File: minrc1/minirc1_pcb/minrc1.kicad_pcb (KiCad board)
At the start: 2 copper layers, 39 x 49.5 mm, 18 parts, among them J3 Conn_01x04, J4 Conn_01x04, U1 DRV8837D, U2 DRV8837D, U3 DRV8837D, U4 DRV8837D, U5 ESP32S3

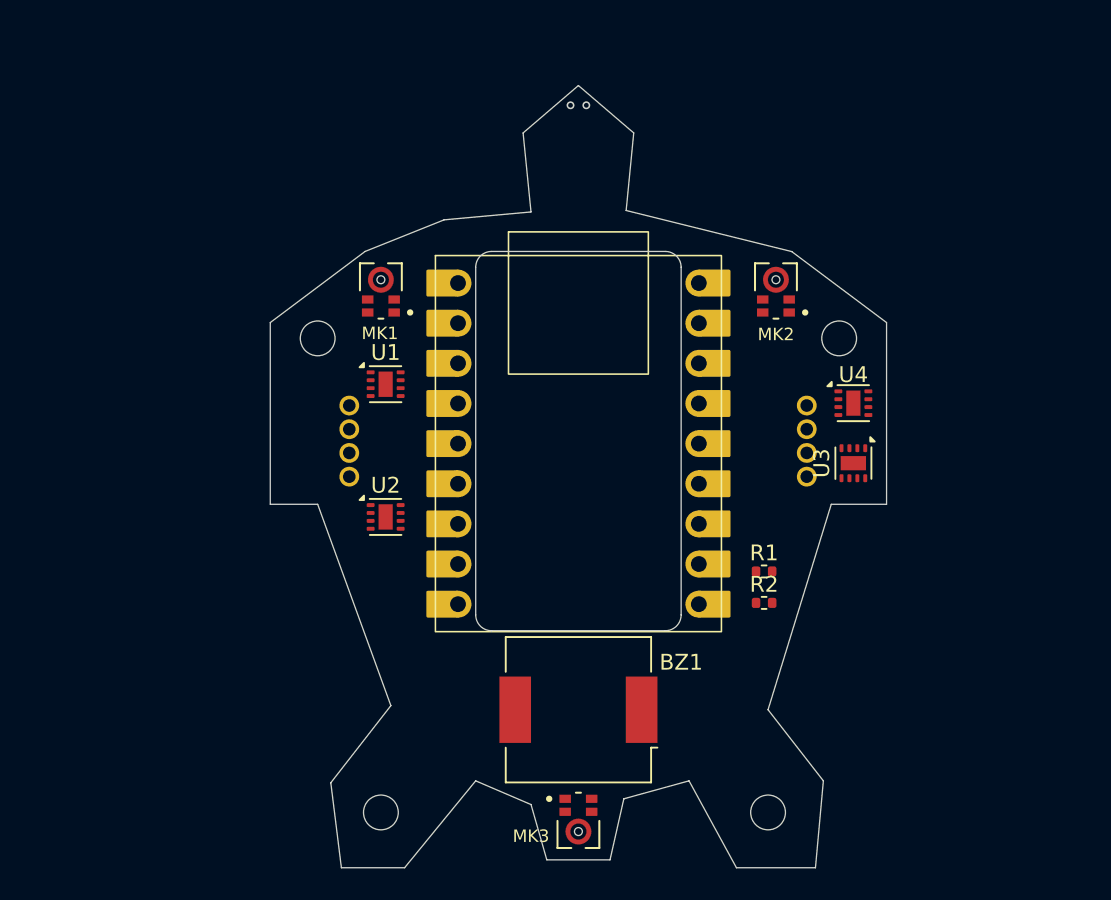
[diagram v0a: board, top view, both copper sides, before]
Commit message: finish turtlebot
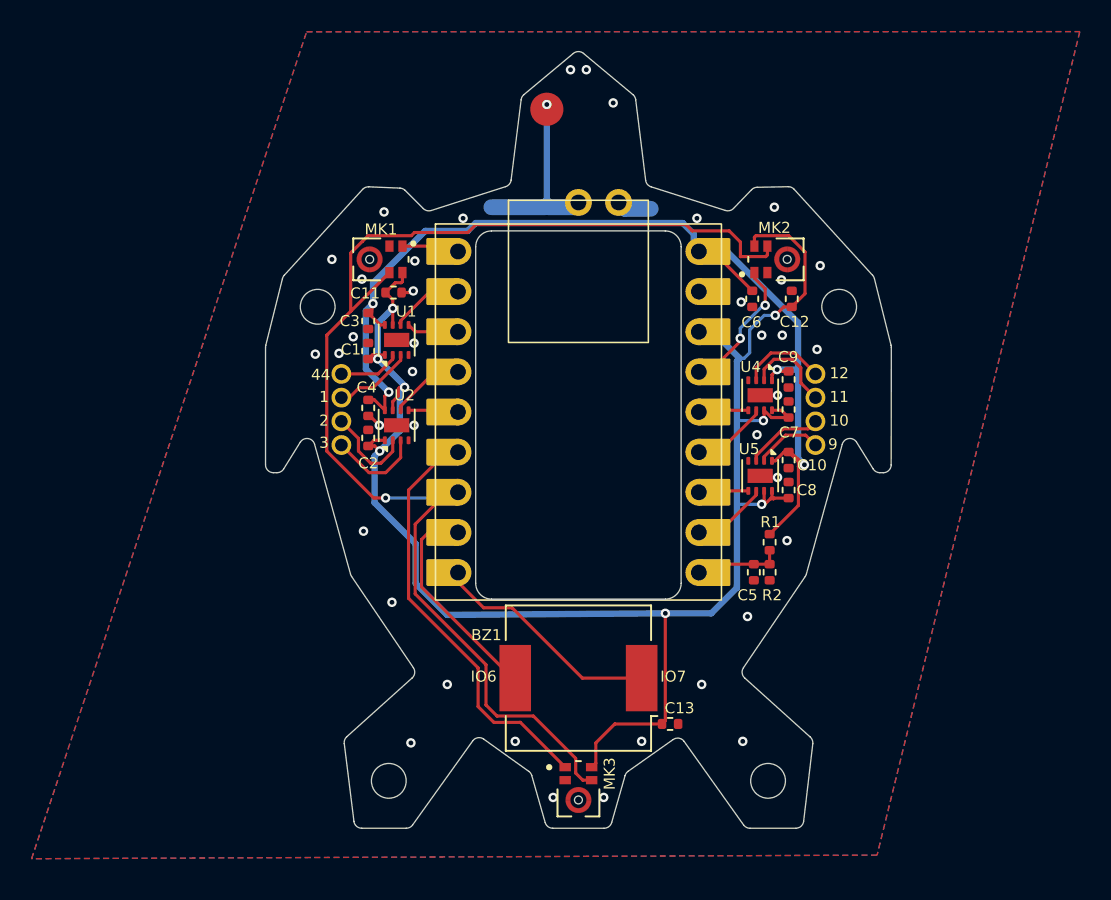
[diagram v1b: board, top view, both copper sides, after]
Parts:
- added C1: 0.1uF, Resistor_SMD:R_0402_1005Metric, F.Cu at (136.7, 106.3)
- added C10: 0.1uF, Resistor_SMD:R_0402_1005Metric, F.Cu at (163.3, 113.2)
- added C11: 0.1uF, Resistor_SMD:R_0402_1005Metric, F.Cu at (138.3, 102.6)
- added C12: 0.1uF, Resistor_SMD:R_0402_1005Metric, F.Cu at (163.5, 103.0)
- added C13: 0.1uF, Resistor_SMD:R_0402_1005Metric, F.Cu at (155.8, 129.9)
- added C2: 0.1uF, Resistor_SMD:R_0402_1005Metric, F.Cu at (136.7, 111.8)
- added C3: 0.1uF, Resistor_SMD:R_0402_1005Metric, F.Cu at (136.7, 104.4)
- added C4: 0.1uF, Resistor_SMD:R_0402_1005Metric, F.Cu at (136.7, 109.9)
- added C5: 0.1uF, Resistor_SMD:R_0402_1005Metric, F.Cu at (161.1, 120.3)
- added C6: 10uF, Resistor_SMD:R_0402_1005Metric, F.Cu at (161.0, 103.0)
- added C7: 0.1uF, Resistor_SMD:R_0402_1005Metric, F.Cu at (163.3, 110.0)
- added C8: 0.1uF, Resistor_SMD:R_0402_1005Metric, F.Cu at (163.3, 115.1)
- added C9: 0.1uF, Resistor_SMD:R_0402_1005Metric, F.Cu at (163.3, 108.1)
- added J4: Switch, Connector_PinHeader_2.54mm:PinHeader_1x02_P2.54mm_Vertical, B.Cu at (150.0, 96.9)
- moved U5 7.48 mm to (161.5, 114.2), turned to -90 degrees
- moved U4 7.30 mm to (161.5, 109.1)
- moved U2 5.84 mm to (138.5, 111.0), turned to 90 degrees
- moved U1 2.89 mm to (138.5, 105.6), turned to 90 degrees
- moved J2 2.07 mm to (165.0, 110.0)
- moved H3 2.06 mm to (138.0, 133.5)
- moved J1 2.06 mm to (135.0, 110.0)
- moved BZ1 2.00 mm to (150.0, 127.0)
- moved H1 2.00 mm to (133.5, 103.5)
- moved H2 2.00 mm to (166.5, 103.5)
- moved H4 2.00 mm to (162.0, 133.5)
- moved MK1 2.00 mm to (137.5, 100.5), turned to -90 degrees
- moved MK2 2.00 mm to (162.5, 100.5), turned to 90 degrees
- moved MK3 2.00 mm to (150.0, 134.0)
- moved U3 2.00 mm to (150.0, 100.0)
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- renumbered J3 to J1, J4 to J2, U5 to U3, U3 to U4, U4 to U5
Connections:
- J2 pad 1: Net-(J4-Pin_1) -> Net-(J2-Pin_1)
- J2 pad 2: Net-(J4-Pin_2) -> Net-(J2-Pin_2)
- J2 pad 3: Net-(J4-Pin_3) -> Net-(J2-Pin_3)
- J2 pad 4: Net-(J4-Pin_4) -> Net-(J2-Pin_4)
- U3 pad 1: Net-(U1-IN1) -> /mic_data1
- U3 pad 11: Net-(U4-IN2) -> Net-(U3-GPIO9)
- U3 pad 12: Net-(U4-IN1) -> Net-(U3-GPIO10)
- U3 pad 13: Net-(U3-IN2) -> Net-(U3-GPIO11)
- U3 pad 14: Net-(U3-IN1) -> Net-(U3-GPIO12)
- U3 pad 2: Net-(U1-IN2) -> Net-(U1-IN1)
- U3 pad 3: Net-(U2-IN1) -> Net-(U1-IN2)
- U3 pad 4: Net-(U2-IN2) -> Net-(U2-IN1)
- U3 pad 5: Net-(BZ1--) -> Net-(U2-IN2)
- U3 pad 6: Net-(BZ1-+) -> /mic_data3
- U3 pad 7: /mic_data1 -> /mic_clk
- U3 pad 8: /mic_data3 -> Net-(BZ1--)
- U3 pad 9: /mic_clk -> Net-(BZ1-+)
- U4 pad 2: Net-(J4-Pin_1) -> Net-(J2-Pin_3)
- U4 pad 3: Net-(J4-Pin_2) -> Net-(J2-Pin_4)
- U4 pad 5: Net-(U3-IN2) -> Net-(U3-GPIO12)
- U4 pad 6: Net-(U3-IN1) -> Net-(U3-GPIO11)
- U5 pad 2: Net-(J4-Pin_3) -> Net-(J2-Pin_1)
- U5 pad 3: Net-(J4-Pin_4) -> Net-(J2-Pin_2)
- U5 pad 5: Net-(U4-IN2) -> Net-(U3-GPIO10)
- U5 pad 6: Net-(U4-IN1) -> Net-(U3-GPIO9)
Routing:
- net +3.3V: track 0.00 -> 113.0 mm, vias 0 -> 8
- net /mic_clk: track 0.00 -> 81.5 mm, vias 0 -> 1
- net VBUS: track 0.00 -> 69.7 mm, vias 0 -> 4
- net /mic_data3: track 0.00 -> 26.7 mm
- net Net-(BZ1-+): track 0.00 -> 14.7 mm
- net Net-(BZ1--): track 0.00 -> 13.8 mm
- net /BATT+: track 0.00 -> 11.9 mm, vias 0 -> 1
- net /mic_data2: track 0.00 -> 9.94 mm, vias 0 -> 2
- net Net-(J1-Pin_4): track 0.00 -> 5.97 mm
- net Net-(J1-Pin_3): track 0.00 -> 5.83 mm
- net Net-(J2-Pin_3): track 0.00 -> 5.77 mm
- net Net-(U3-GPIO8): track 0.00 -> 5.58 mm
- net Net-(J2-Pin_4): track 0.00 -> 5.50 mm
- net Net-(J2-Pin_2): track 0.00 -> 4.98 mm
- net Net-(U3-GPIO11): track 0.00 -> 4.88 mm
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- added copper zone on B.Cu, net GND
- added copper zone on F.Cu, net GND
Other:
- board size 39 x 49.5 mm -> 39.6 x 49.1 mm
- board text added: "1"
- board text added: "10"
- board text added: "11"
- board text added: "12"
- board text added: "2"
- board text added: "3"
- board text added: "44"
- board text added: "9"
- board text added: "IO6"
- board text added: "IO7"
- board text added: "OFF"
- board text added: "ON"
- board text added: "bat+"
- board text added: "by Chris Xu"
- board text added: "chrg"
- board text added: "minirc1"

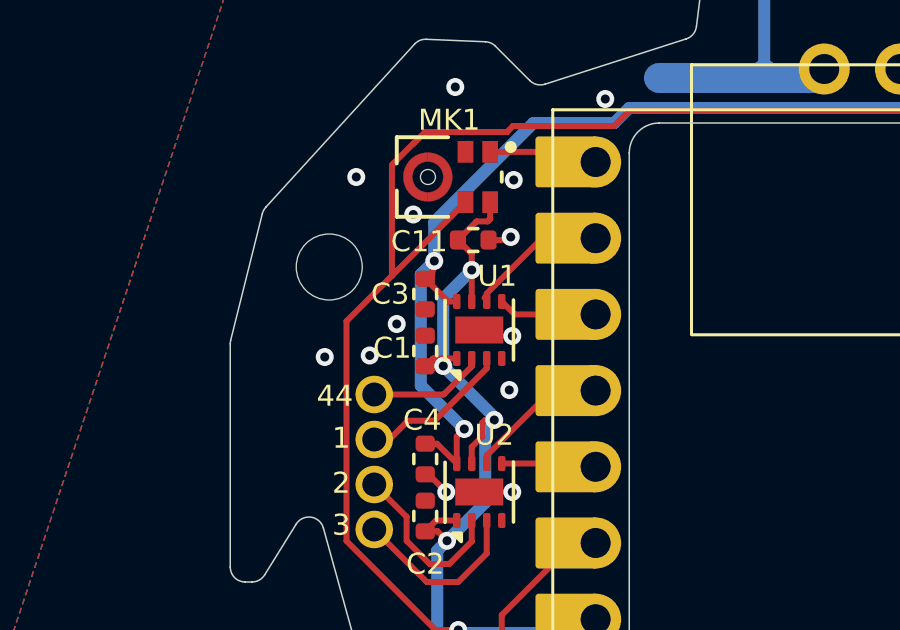
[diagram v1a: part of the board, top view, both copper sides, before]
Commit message: update readme
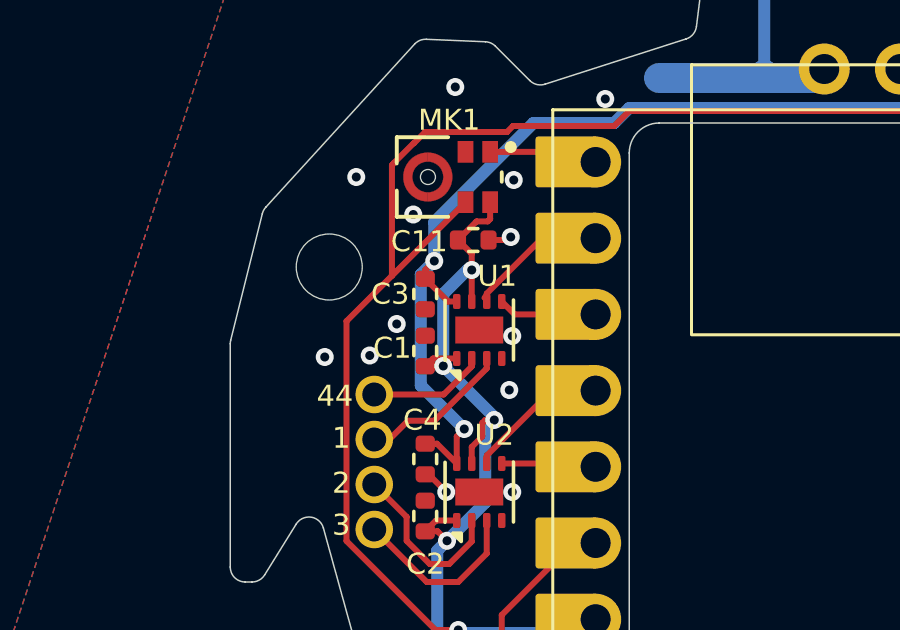
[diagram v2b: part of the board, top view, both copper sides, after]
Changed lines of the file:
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@@
 	)
 	(segment
-		(start 137.3 104.55)
-		(end 138.25 103.6)
+		(start 137.3 104.4)
+		(end 138.1 103.6)
 		(width 0.4)
 		(layer "B.Cu")
@@
 	)
 	(segment
+		(start 138.1 103.6)
+		(end 138.25 103.6)
+		(width 0.4)
+		(layer "B.Cu")
+		(net "+3.3V")
+	)
+	(segment
 		(start 157.62 105.08)
 		(end 158.518144 105.08)
@@
 	)
 	(segment
-		(start 137.3 106.8)
-		(end 137.3 104.55)
-		(width 0.4)
-		(layer "B.Cu")
-		(net "+3.3V")
-	)
-	(segment
 		(start 160.03 121.13)
 		(end 160.033879 121.133879)
@@
 	)
 	(segment
+		(start 137.3 106.8)
+		(end 137.3 104.4)
+		(width 0.4)
+		(layer "B.Cu")
+		(net "+3.3V")
+	)
+	(segment
 		(start 155.5 122.9)
 		(end 158.40918 122.9)
@@
 	)
 	(segment
-		(start 136.91 103.89)
-		(end 136.7 103.89)
-		(width 0.2)
-		(layer "F.Cu")
-		(net "VBUS")
-	)
-	(segment
 		(start 137.46 104.65)
 		(end 136.7 103.89)
@@
 	(segment
 		(start 137 103.3)
-		(end 136.91 103.89)
+		(end 136.7 103.6)
 		(width 0.2)
 		(layer "F.Cu")
@@
 	)
 	(segment
+		(start 136.7 103.6)
+		(end 136.7 103.89)
+		(width 0.2)
+		(layer "F.Cu")
+		(net "VBUS")
+	)
+	(segment
 		(start 137.09 109.39)
 		(end 137.75 110.05)
@@
 	)
 	(segment
+		(start 136.55 107.45)
+		(end 136.55 103.75)
+		(width 0.4)
+		(layer "B.Cu")
+		(net "VBUS")
+	)
+	(segment
 		(start 163.9 107.5)
 		(end 163.9 113.1)
@@
 	)
 	(segment
-		(start 136.55 107.45)
-		(end 136.55 103.75)
-		(width 0.4)
-		(layer "B.Cu")
-		(net "VBUS")
-	)
-	(segment
 		(start 157.3 99.68)
 		(end 157.62 100)
@@
 	)
 	(segment
+		(start 138 108.9)
+		(end 136.55 107.45)
+		(width 0.4)
+		(layer "B.Cu")
+		(net "VBUS")
+	)
+	(segment
 		(start 163.874265 107.474265)
 		(end 163.9 107.5)
@@
 		(width 0.4)
 		(layer "B.Cu")
-		(net "VBUS")
-	)
-	(segment
-		(start 138 108.9)
-		(end 136.55 107.45)
-		(width 0.4)
-		(layer "B.Cu")
